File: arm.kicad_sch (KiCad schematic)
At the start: 37 parts, among them J1 TC2030-IDC-NL, U10 24CW1280T, U4 STM32F103T6U6A, U6 KTD2052, U7 TLT9251VLE, U8 MAX17671FATB+

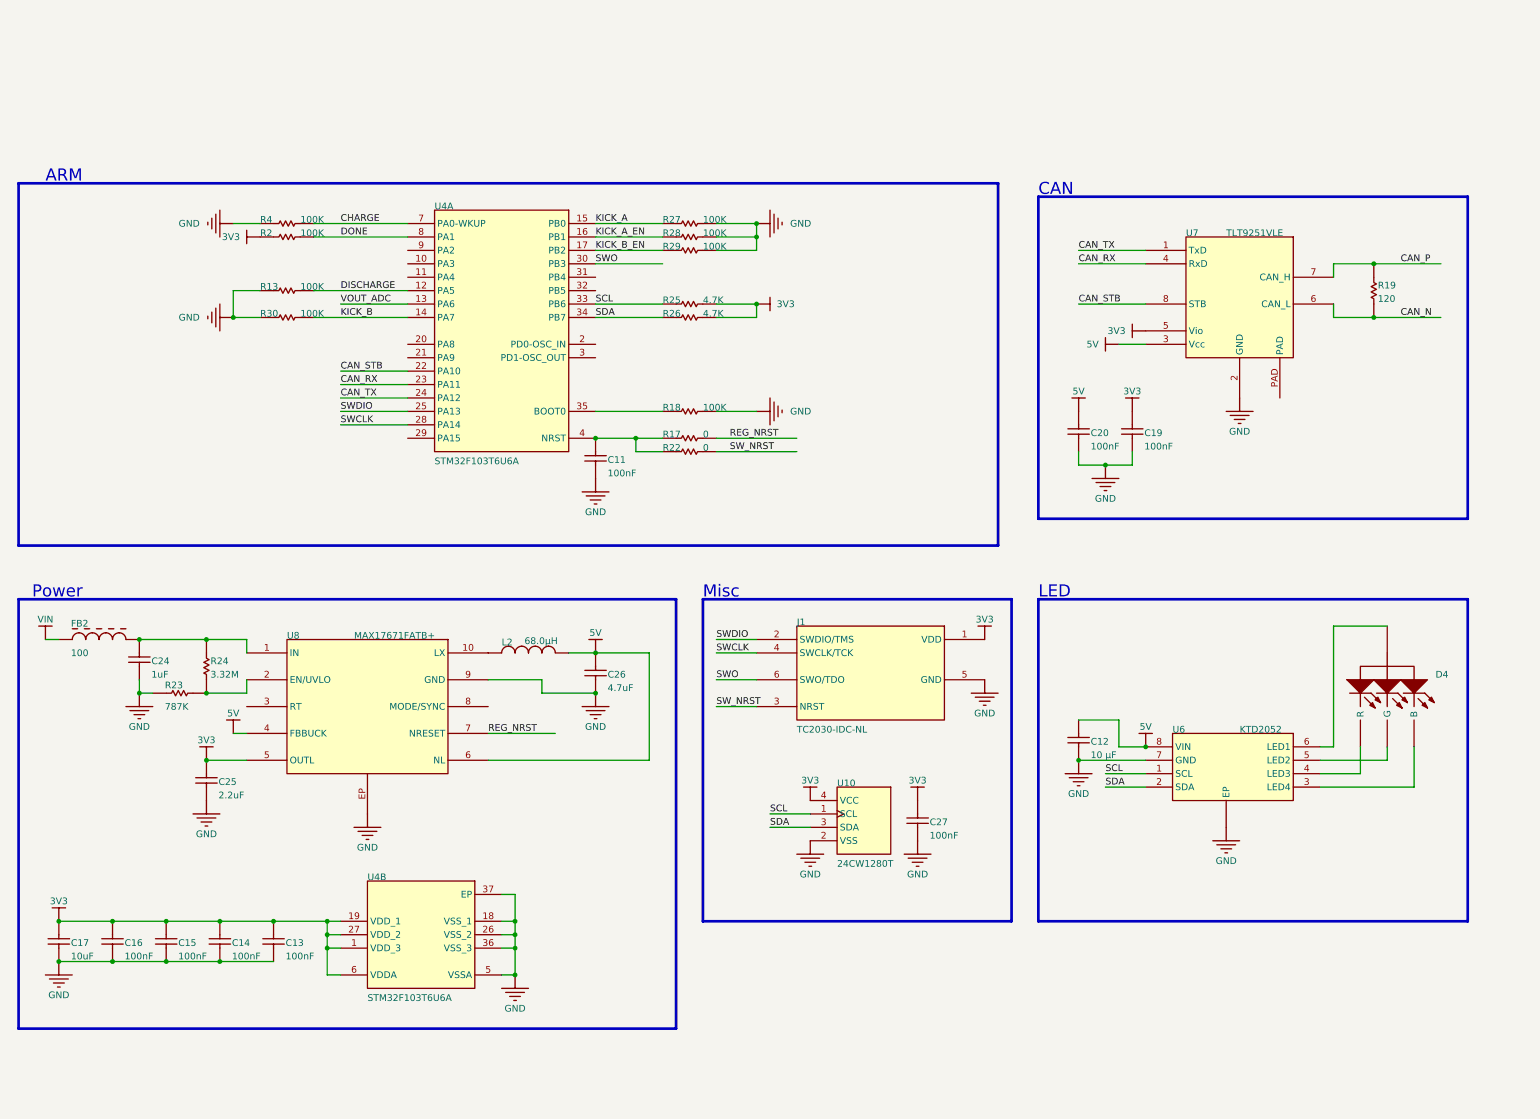
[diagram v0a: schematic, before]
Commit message: Cleanup the project after moving to KiCad.
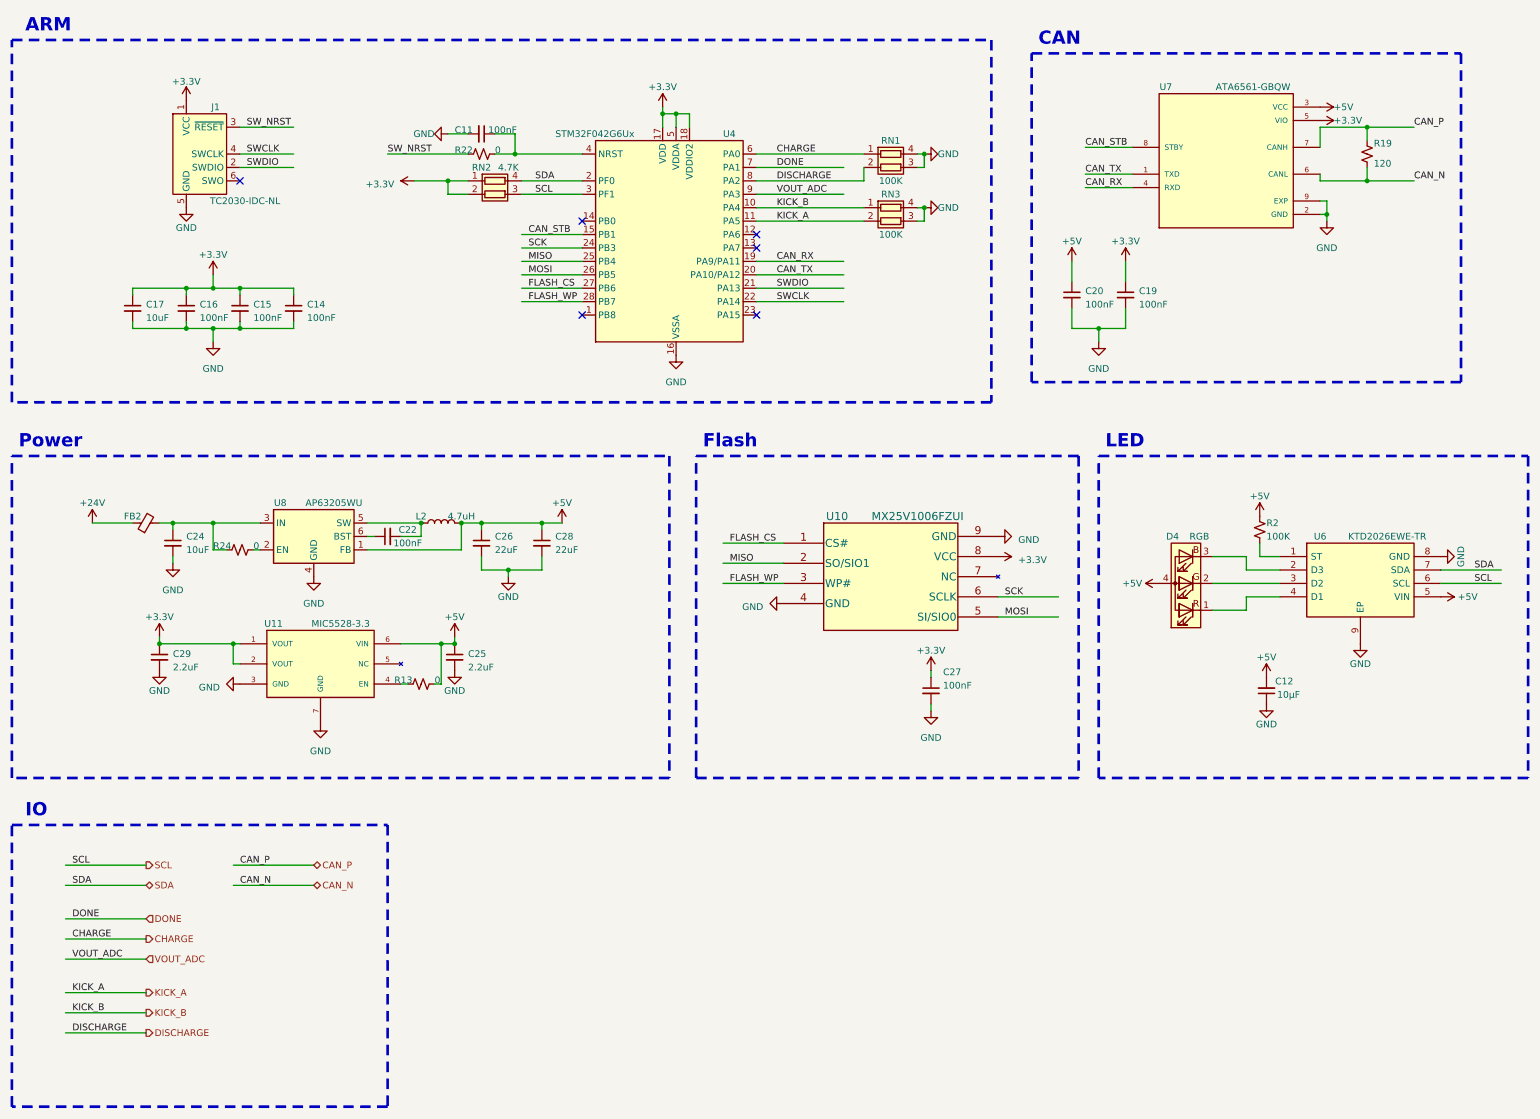
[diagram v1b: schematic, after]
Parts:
- removed C11: 100nF, PCB-lqeomw61a722wi99q4vw-1, symbol mikona-altium-import:1_SYM-773ebe35ab3ba8f9-3
- removed C12: 10 µF, RESC2013X55X40ML15T20, symbol mikona-altium-import:1_SYM-55069f29b9a38ac1-2
- removed C13, C14, C15, C16, C19, C20: 100nF, PCB-ya5qsrmvtd5pjczft90h-1, symbol mikona-altium-import:1_SYM-f7023f833ffb28c5-1
- removed C17: 10uF, PCB-8tuutlkq7p1aj3t2dfdp-1, symbol mikona-altium-import:1_SYM-55c098f4cfa08a07-1
- removed C24: 1uF, CAPC1608X90X35ML15T15, symbol mikona-altium-import:1_SYM-ce7a065e703111bd-1
- removed C25: 2.2uF, CAPC1608X90X35LL10T15, symbol mikona-altium-import:1_CAP-2
- removed C26: 4.7uF, CAPC1608X90X35NL10T15, symbol mikona-altium-import:1_GRM188Z71C475KE21J
- removed D4: Lite-On LTST-C19HE1WT, PCB-52d9enhv62acg8agpph7-1, symbol mikona-altium-import:3_SYM-1946d08468e8c681-4
- removed FB2: 100, MURA-BLM18KG_TN-B60-CHIP-2_V3, symbol mikona-altium-import:0_MURA-FB-2
- removed J1: TC2030-IDC-NL, PCB-ltb50y2q1twco73v61fe-1, symbol mikona-altium-import:0_TC2030-MCP-NL-Symbol-1
- removed L2: 68.0µH, PCB-o31o4oqkad523pnvsppd-1, symbol mikona-altium-import:0_SYM-3019f8d9a4f8efde-1
- removed R13, R2, R27, R28, R29, R30, R4: 100K, RESC1005X40X25ML10T10, symbol mikona-altium-import:0_RES-2
- removed R17: 0, RESC1005X40X25ML05T10, symbol mikona-altium-import:0_RES-2
- removed R18: 100K, RESC1005X40X25ML10T10, symbol mikona-altium-import:2_RES-2
- removed R19: 120, RESC1005X37X25LL05T10, symbol mikona-altium-import:1_RES-2
- removed R22: 0, RESC1005X40X25ML05T10, symbol mikona-altium-import:2_RES-2
- removed R23: 787K, RESC1005X40X25LL05T05, symbol mikona-altium-import:0_RES-2
- removed R24: 3.32M, RESC1005X40X25NL05T05, symbol mikona-altium-import:1_RES-2
- removed R25, R26: 4.7K, RESC1005X40X25NL05T05, symbol mikona-altium-import:0_SYM-e02329a4a0913fe4-1
- removed U10: 24CW1280T, PCB-du7oa82jyfofml92o6ch-1, symbol mikona-altium-import:0_SYM-b1fc7d542f6b6e3b-1
- removed U4: STM32F103T6U6A, STM-VFQFPN36_L, symbol mikona-altium-import:0_MC-ARM-STM32F103X4_6-SQ37
- removed U6: KTD2052, PCB-1zdkv4te5dlcf1e3m0hc-1, symbol mikona-altium-import:0_KTD2052
- removed U7: TLT9251VLE, PCB-is4r40753zstvrjiqh7i-1, symbol mikona-altium-import:0_Infineon TLT9251VLEXUMA1-Symbol-1
- removed U8: MAX17671FATB+, T1033+1_V, symbol mikona-altium-import:0_Maxim Integrated MAX17671FATB+
- added C11, C14, C15, C16, C19, C20, C22: 100nF, Capacitor_SMD:C_0402_1005Metric_Pad0.74x0.62mm_HandSolder, symbol Device:C_Small
- added C12: 10µF, Capacitor_SMD:C_0805_2012Metric_Pad1.18x1.45mm_HandSolder, symbol Device:C_Small
- added C17: 10uF, Capacitor_SMD:C_0402_1005Metric_Pad0.74x0.62mm_HandSolder, symbol Device:C_Small
- added C24: 10uF, Capacitor_SMD:C_0603_1608Metric_Pad1.08x0.95mm_HandSolder, symbol Device:C_Small
- added C25, C29: 2.2uF, Capacitor_SMD:C_0402_1005Metric_Pad0.74x0.62mm_HandSolder, symbol Device:C_Small
- added C26, C28: 22uF, Capacitor_SMD:C_0805_2012Metric_Pad1.18x1.45mm_HandSolder, symbol Device:C_Small
- added D4: RGB, LED_SMD:LED_LiteOn_LTST-C19HE1WT, symbol Device:LED_RGBA
- added FB2: FerriteBead_Small, Resistor_SMD:R_0603_1608Metric_Pad0.98x0.95mm_HandSolder, symbol Device:FerriteBead_Small
- added J1: TC2030-IDC-NL, Connector:Tag-Connect_TC2030-IDC-NL_2x03_P1.27mm_Vertical, symbol Connector:Conn_ARM_SWD_TagConnect_TC2030-NL
- added L2: 4.7uH, Inductor_SMD:L_Taiyo-Yuden_NR-50xx_HandSoldering, symbol Device:L
- added R13, R22, R24: 0, Resistor_SMD:R_0402_1005Metric_Pad0.72x0.64mm_HandSolder, symbol Device:R_Small_US
- added R19: 120, Resistor_SMD:R_0402_1005Metric_Pad0.72x0.64mm_HandSolder, symbol Device:R_Small_US
- added R2: 100K, Resistor_SMD:R_0402_1005Metric_Pad0.72x0.64mm_HandSolder, symbol Device:R_Small_US
- added RN1, RN3: 100K, Resistor_SMD:R_Array_Convex_2x0402, symbol Device:R_Pack02
- added RN2: 4.7K, Resistor_SMD:R_Array_Convex_2x0402, symbol Device:R_Pack02
- added U10: MX25V1006FZUI, MX25V1006FZUI:MX25V1006FZUI, symbol MX25V1006FZUI:MX25V1006FZUI
- added U11: MIC5528-3.3, MIC5528-3.3YMT-TR:SON40P120X120X60-7N, symbol MIC5528-3.3YMT-TR:MIC5528-3.3YMT-TR
- added U4: STM32F042G6Ux, Package_DFN_QFN:QFN-28_4x4mm_P0.5mm, symbol MCU_ST_STM32F0:STM32F042G6Ux
- added U6: KTD2026EWE-TR, KTD2026EWE-TR:SON40P150X150X55-9N, symbol KTD2026EWE-TR:KTD2026EWE-TR
- added U7: ATA6561-GBQW, ATA6561-GBQW:SON65P300X300X100-9N, symbol ATA6561-GBQW:ATA6561-GBQW
- added U8: AP63205WU, Package_TO_SOT_SMD:TSOT-23-6, symbol Regulator_Switching:AP63205WU
- C27: footprint PCB-ya5qsrmvtd5pjczft90h-1 -> Capacitor_SMD:C_0402_1005Metric_Pad0.74x0.62mm_HandSolder; symbol mikona-altium-import:1_SYM-f7023f833ffb28c5-1 -> Device:C_Small
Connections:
- net 3V3 is gone; now on net GND: C27.2
- net CAN_N: now also R19.2, U7.6 (CANL)
- net CAN_P: now also R19.1, U7.7 (CANH)
- net CAN_RX: now also U4.19 (PA9/PA11), U7.4 (RXD)
- net CAN_STB: now also U4.15 (PB1), U7.8 (STBY)
- net CAN_TX: now also U4.20 (PA10/PA12), U7.1 (TXD)
- net CHARGE: now also RN1.1 (R1.1), U4.6 (PA0)
- net DISCHARGE: now also RN1.2 (R2.1), U4.8 (PA2)
- net DONE: now also U4.7 (PA1)
- net GND: now also C11.2, C12.1, C14.2, C15.2, C16.2, C17.2, C19.2, C20.2, C24.2, C25.2, C26.2, C28.2, C29.2, J1.5 (GND), RN1.3 (R2.2), RN1.4 (R1.2), RN3.3 (R2.2), RN3.4 (R1.2), U10.4 (GND), U10.9 (GND), U11.3 (GND), U11.7 (GND), U4.16 (VSSA), U6.8 (GND), U6.9 (EP), U7.2 (GND), U7.9 (EXP), U8.4 (GND); no longer C27.1
- net KICK_A: now also RN3.2 (R2.1), U4.11 (PA5)
- net KICK_B: now also RN3.1 (R1.1), U4.10 (PA4)
- net SCL: now also RN2.3 (R2.2), U4.3 (PF1), U6.6 (SCL)
- net SDA: now also RN2.4 (R1.2), U4.2 (PF0), U6.7 (SDA)
- net SWCLK: now also J1.4 (SWCLK), U4.22 (PA14)
- net SWDIO: now also J1.2 (SWDIO), U4.21 (PA13)
- net SW_NRST: now also J1.3 (~{RESET}), R22.2
- net VOUT_ADC: now also U4.9 (PA3)
- new net: R2.2, U6.1 (ST)
- new net: D4.3 (BK), U6.2 (D3)
- new net: D4.2 (GK), U6.3 (D2)
- new net: D4.1 (RK), U6.4 (D1)
- new net: C24.1, FB2.2, R24.2, U8.3 (IN)
- new net: C11.1, R22.1, U4.4 (NRST)
- new net: R24.1, U8.2 (EN)
- new net: C22.2, L2.1, U8.5 (SW)
- new net: C22.1, U8.6 (BST)
- new net: R13.2, U11.4 (EN)
- new net +24V: FB2.1
- new net +3.3V: C14.1, C15.1, C16.1, C17.1, C19.1, C27.1, C29.1, J1.1 (VCC), RN2.1 (R1.1), RN2.2 (R2.1), U10.8 (VCC), U11.1 (VOUT), U11.2 (VOUT), U4.17 (VDD), U4.18 (VDDIO2), U4.5 (VDDA), U7.5 (VIO)
- new net +5V: C12.2, C20.1, C25.1, C26.1, C28.1, D4.4 (A), L2.2, R13.1, R2.1, U11.6 (VIN), U6.5 (VIN), U7.3 (VCC), U8.1 (FB)
- new net FLASH_CS: U10.1 (CS#), U4.27 (PB6)
- new net FLASH_WP: U10.3 (WP#), U4.28 (PB7)
- new net MISO: U10.2 (SO/SIO1), U4.25 (PB4)
- new net MOSI: U10.5 (SI/SIO0), U4.26 (PB5)
- new net SCK: U10.6 (SCLK), U4.24 (PB3)
- no-connect marks 0 -> 6
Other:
- note added: "Flash"
- note added: "IO"
- note removed: "Misc"
